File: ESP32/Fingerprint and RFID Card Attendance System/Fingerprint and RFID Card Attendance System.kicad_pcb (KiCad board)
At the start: 2 copper layers, 97.4 x 137.5 mm, 63 parts, among them J1 RTC, J11 V_OUT, J12 +BATT, J13 BUTTONS, J14 AS608, J15 SD MODULE, J16 -BATT, J17 SW_C, J18 SW_NO, J2 SCREEN, J3 +5V_IN, J4 -5V_OUT, J5 +5V_IN, J6 -5V_IN, J9 +UPS, Q1 2SC1815, U1 ESP32-S3-DEVKITC-1-N8R8, U2 LM2596S-3.3V, U3 RC522

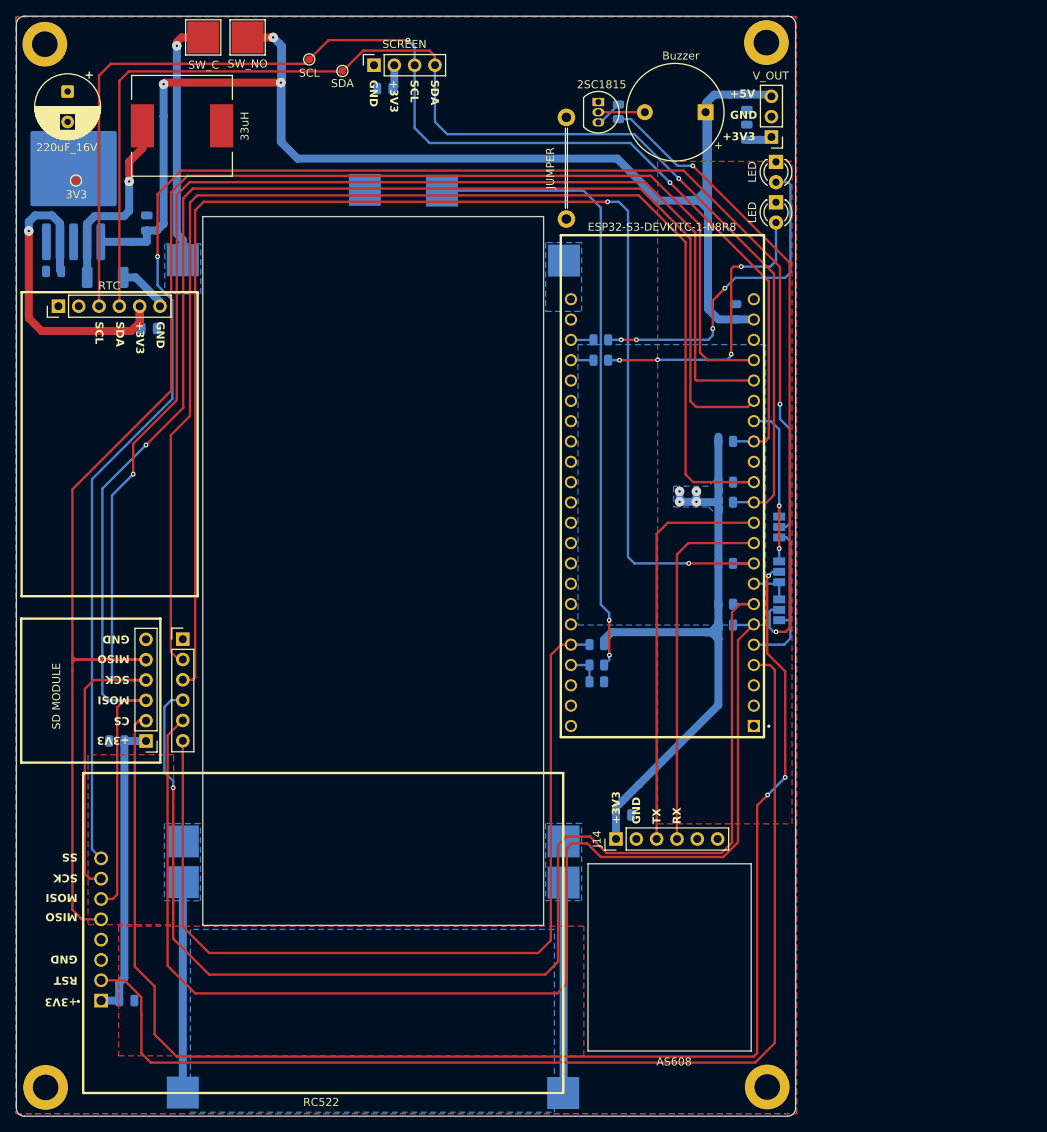
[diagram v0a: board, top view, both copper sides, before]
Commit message: Updates from Work
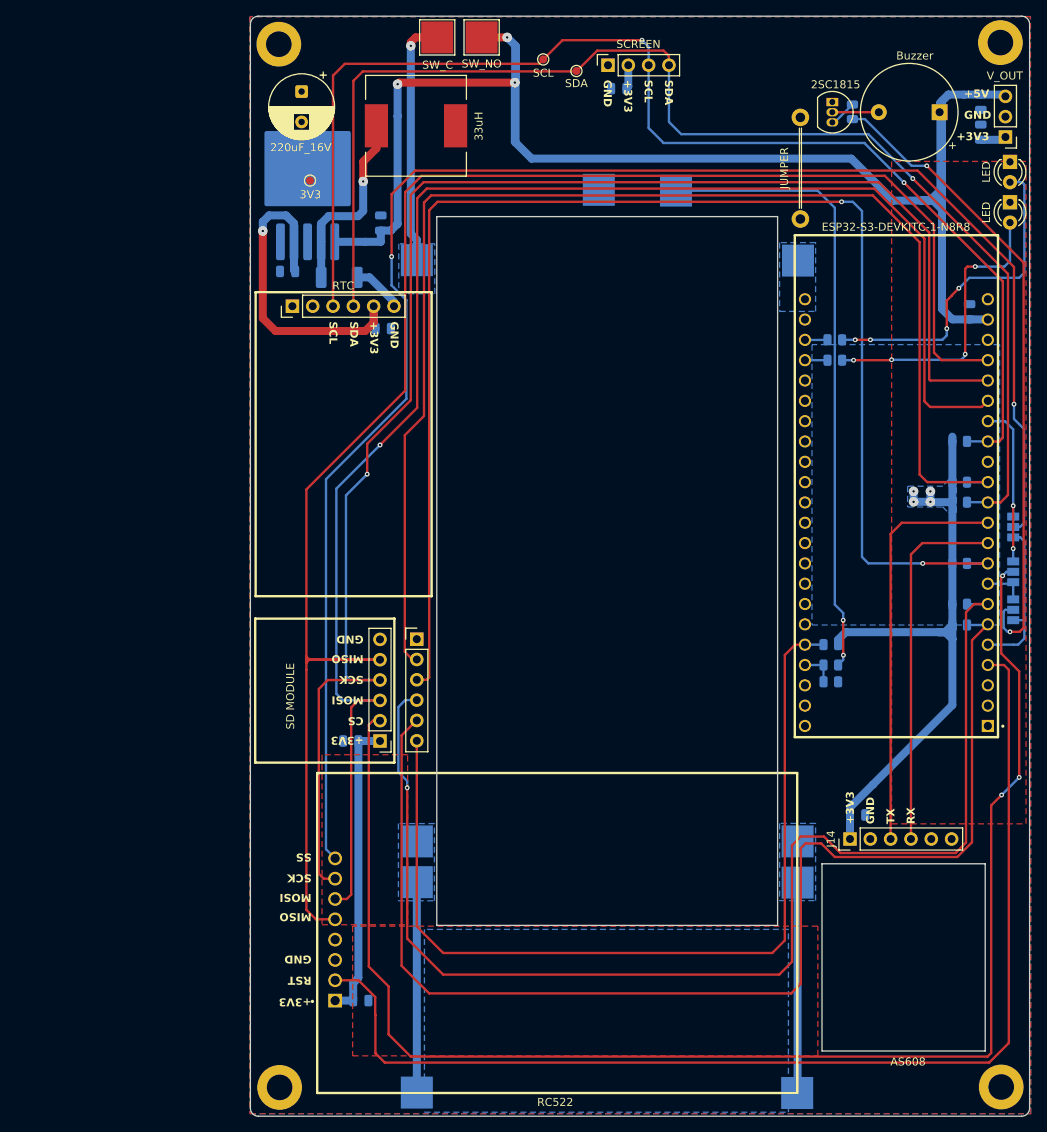
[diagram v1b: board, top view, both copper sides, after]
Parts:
- moved R11 29.3 mm to (145.8, 106.4)
- moved R3 29.3 mm to (146.3, 68.3)
- moved R4 29.3 mm to (146.3, 70.8)
- moved R5 29.3 mm to (145.8, 109.0)
- moved R6 29.3 mm to (145.8, 111.0)
- moved C8 29.3 mm to (77.9, 59.8)
- moved U2 29.3 mm to (80.4, 48.4)
- moved 3.3V5 29.2 mm to (80.7, 48.4)
- moved 5V1 29.2 mm to (106.4, 42.6)
- moved BZ1 29.2 mm to (159.4, 39.9)
- moved C1 29.2 mm to (119.3, 36.9)
- moved C10 29.2 mm to (149.2, 127.7)
- moved C11 29.2 mm to (85.8, 118.5)
- moved C3 29.2 mm to (163.2, 64.8)
- moved C4 29.2 mm to (89.5, 53.7)
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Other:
- outline, holes or cut-outs redrawn
